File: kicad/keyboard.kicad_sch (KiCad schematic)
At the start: 169 parts, among them SW1 Push, SW10 Push, SW11 Push, SW12 Push, SW13 Push, SW14 Push, SW15 Push, SW16 Push, SW17 Push, SW18 Push, SW19 Push, SW2 Push, SW20 Push, SW21 Push, SW22 Push, SW23 Push, SW24 Push, SW25 Push, SW26 Push, SW27 Push, SW28 Push, SW29 Push, SW3 Push, SW30 Push, SW31 Push, SW32 Push, SW33 Push, SW34 Push, SW35 Push, SW36 Push, SW37 Push, SW38 Push, SW39 Push, SW4 Push, SW40 Push, SW41 Push, SW42 Push, SW43 Push, SW44 Push, SW45 Push, SW46 Push, SW47 Push, SW48 Push, SW49 Push, SW5 Push, SW50 Push, SW51 Push, SW52 Push, SW53 Push, SW54 Push, SW55 Push, SW56 Push, SW57 Push, SW58 Push, SW59 Push, SW6 Push, SW60 Push, SW61 Push, SW62 Push, SW63 Push, SW64 Push, SW65 Push, SW66 Push, SW67 Push, SW68 Push, SW69 Push, SW7 Push, SW70 Push, SW71 Push, SW72 Push, SW73 Push, SW74 Push, SW75 Push, SW76 Push, SW77 Push, SW78 Push, SW79 Push, SW8 Push, SW80 Push, SW81 Push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

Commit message: 2
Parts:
- D1, D10, D11, D12, D13, D14, D15, D16, D17, D18, D19, D2, D20, D21, D22, D23, D24, D25, D26, D27, D28, D29, D3, D30, D31, D32, D33, D34, D35, D36, D37, D38, D39, D4, D40, D41, D42, D43, D44, D45, D46, D47, D48, D49, D5, D50, D51, D52, D53, D54, D55, D56, D57, D58, D59, D6, D60, D61, D62, D63, D64, D65, D66, D67, D68, D69, D7, D70, D71, D72, D73, D74, D75, D76, D77, D78, D79, D8, D80, D81, D82, D83, D84, D9: footprint MyLibrary:D1206 -> ScottoKeebs_Components:Diode_SOD-123
- SW1, SW10, SW11, SW12, SW13, SW14, SW15, SW16, SW17, SW18, SW19, SW2, SW20, SW21, SW22, SW23, SW24, SW25, SW26, SW27, SW28, SW29, SW3, SW30, SW31, SW32, SW33, SW34, SW35, SW36, SW37, SW38, SW39, SW4, SW40, SW41, SW42, SW43, SW44, SW45, SW46, SW47, SW48, SW49, SW5, SW50, SW51, SW52, SW53, SW54, SW55, SW56, SW57, SW58, SW59, SW6, SW60, SW61, SW62, SW63, SW64, SW65, SW66, SW67, SW68, SW69, SW7, SW70, SW71, SW72, SW73, SW74, SW75, SW76, SW77, SW78, SW79, SW8, SW80, SW81, SW82, SW83, SW84, SW9: footprint Library:Kailh_socket_PG1350 -> Gateron_KS33_Solderable:Gateron-KS33-Solderable-1U

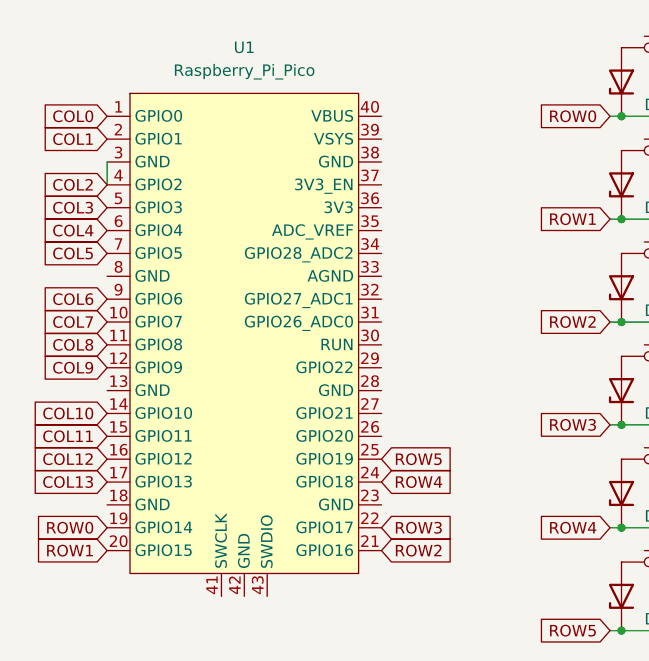
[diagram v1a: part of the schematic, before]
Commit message: pi traces
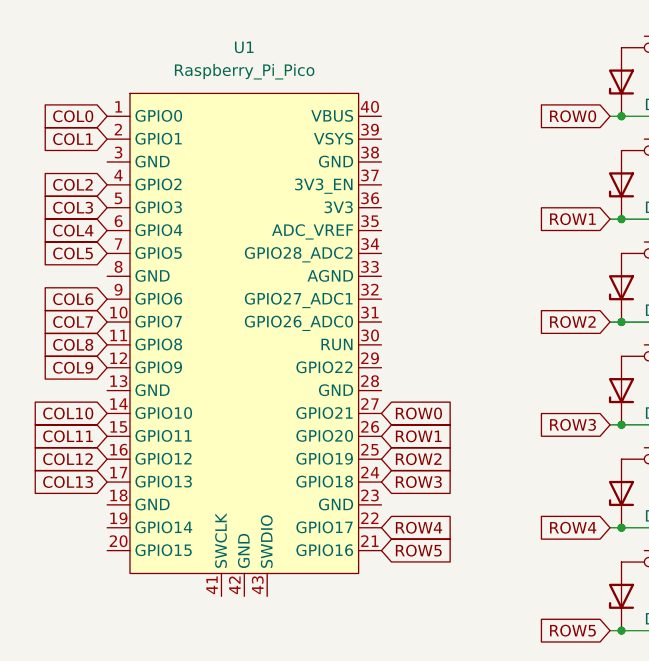
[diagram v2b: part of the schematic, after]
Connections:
- net COL2: no longer U1.3 (GND)
- net ROW0: now also U1.27 (GPIO21); no longer U1.19 (GPIO14)
- net ROW1: now also U1.26 (GPIO20); no longer U1.20 (GPIO15)
- net ROW2: now also U1.25 (GPIO19); no longer U1.21 (GPIO16)
- net ROW3: now also U1.24 (GPIO18); no longer U1.22 (GPIO17)
- net ROW4: now also U1.22 (GPIO17); no longer U1.24 (GPIO18)
- net ROW5: now also U1.21 (GPIO16); no longer U1.25 (GPIO19)
